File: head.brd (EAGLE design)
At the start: 15.5 x 13.2 mm, 6 parts

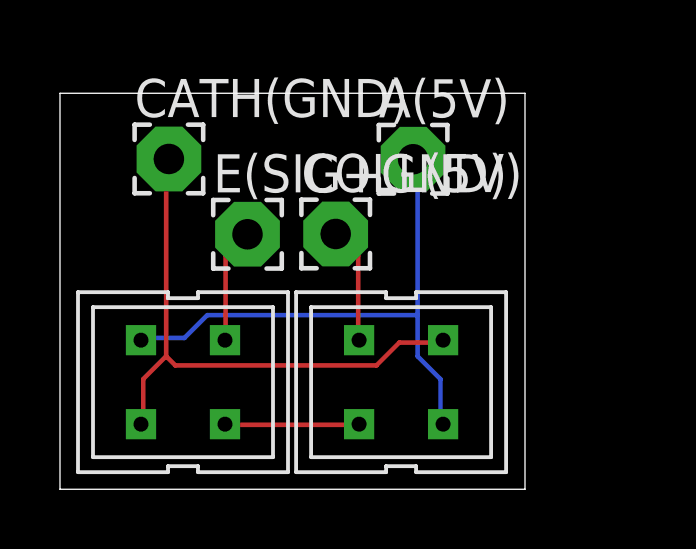
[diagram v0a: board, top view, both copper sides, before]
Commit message: no message
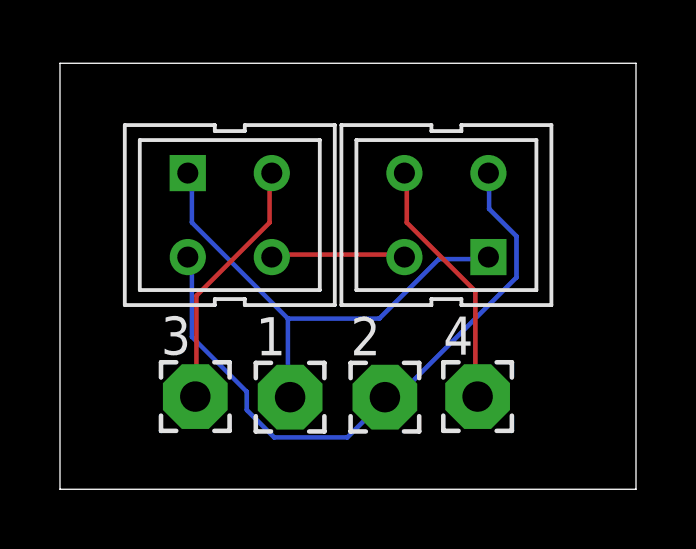
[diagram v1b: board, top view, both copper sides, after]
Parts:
- removed A(5V), CATH(GND), COLL(5V), E(SIG+GND): (no value), wirepad:2,15/1,0
- added 1, 2, 3, 4: (no value), wirepad:2,15/1,0
- moved U$2 5.78 mm to (5.66, 9.14)
- moved U$1 5.77 mm to (12.9, 9.14)
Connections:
- net A(5V): now also 1.1; no longer A(5V).1
- net CATH(GND): now also 2.1; no longer CATH(GND).1
- net COLL(5V): now also 4.1; no longer COLL(5V).1
- net E(SIG+GND): now also 3.1; no longer E(SIG+GND).1
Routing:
- net E(SIG+GND): track 3.84 -> 8.51 mm
- net COLL(5V): track 3.87 -> 8.49 mm
- net CATH(GND): track 19.0 -> 21.4 mm
- net A(5V): track 18.9 -> 16.4 mm
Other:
- board size 15.5 x 13.2 mm -> 19.2 x 14.2 mm
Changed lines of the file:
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@@
 <setting verticaltext="up"/>
 </settings>
-<grid distance="0.1" unitdist="mm" unit="mm" style="lines" multiple="1" display="yes" altdistance="1" altunitdist="mm" altunit="mm"/>
+<grid distance="0.1" unitdist="mm" unit="mm" style="lines" multiple="1" display="yes" altdistance="0.1" altunitdist="mm" altunit="mm"/>
 <layers>
 <layer number="1" name="Top" color="4" fill="1" visible="yes" active="yes"/>
@@
 <layer number="43" name="vRestrict" color="2" fill="10" visible="yes" active="yes"/>
 <layer number="44" name="Drills" color="7" fill="1" visible="no" active="yes"/>
-<layer number="45" name="Holes" color="7" fill="1" visible="yes" active="yes"/>
+<layer number="45" name="Holes" color="7" fill="1" visible="no" active="yes"/>
 <layer number="46" name="Milling" color="3" fill="1" visible="no" active="yes"/>
 <layer number="47" name="Measures" color="7" fill="1" visible="no" active="yes"/>
@@
 <board>
 <plain>
-<wire x1="0" y1="0" x2="15.5" y2="0" width="0" layer="20"/>
-<wire x1="15.5" y1="0" x2="15.5" y2="13.2" width="0" layer="20"/>
-<wire x1="15.5" y1="13.2" x2="0" y2="13.2" width="0" layer="20"/>
-<wire x1="0" y1="13.2" x2="0" y2="0" width="0" layer="20"/>
+<wire x1="0" y1="0" x2="19.2" y2="0" width="0" layer="20"/>
+<wire x1="19.2" y1="0" x2="19.2" y2="14.2" width="0" layer="20"/>
+<wire x1="19.2" y1="14.2" x2="0" y2="14.2" width="0" layer="20"/>
+<wire x1="0" y1="14.2" x2="0" y2="0" width="0" layer="20"/>
 </plain>
 <attributes>
@@
 </autorouter>
 <elements>
-<element name="A(5V)" library="wirepad" library_urn="urn:adsk.eagle:library:412" package="2,15/1,0" package3d_urn="urn:adsk.eagle:package:30831/1" value="" x="11.77" y="11"/>
-<element name="CATH(GND)" library="wirepad" library_urn="urn:adsk.eagle:library:412" package="2,15/1,0" package3d_urn="urn:adsk.eagle:package:30831/1" value="" x="3.63" y="11.01"/>
-<element name="COLL(5V)" library="wirepad" library_urn="urn:adsk.eagle:library:412" package="2,15/1,0" package3d_urn="urn:adsk.eagle:package:30831/1" value="" x="9.19" y="8.51"/>
-<element name="E(SIG+GND)" library="wirepad" library_urn="urn:adsk.eagle:library:412" package="2,15/1,0" package3d_urn="urn:adsk.eagle:package:30831/1" value="" x="6.25" y="8.5"/>
-<element name="U$1" library="ferraris_sensor_project" package="CNY70" value="CNY70" x="11.37" y="3.57" rot="R180"/>
-<element name="U$2" library="ferraris_sensor_project" package="CNY70" value="CNY70" x="4.1" y="3.57"/>
+<element name="1" library="wirepad" library_urn="urn:adsk.eagle:library:412" package="2,15/1,0" package3d_urn="urn:adsk.eagle:package:30831/1" value="" x="7.67" y="3.07"/>
+<element name="2" library="wirepad" library_urn="urn:adsk.eagle:library:412" package="2,15/1,0" package3d_urn="urn:adsk.eagle:package:30831/1" value="" x="10.83" y="3.07"/>
+<element name="3" library="wirepad" library_urn="urn:adsk.eagle:library:412" package="2,15/1,0" package3d_urn="urn:adsk.eagle:package:30831/1" value="" x="4.51" y="3.09"/>
+<element name="4" library="wirepad" library_urn="urn:adsk.eagle:library:412" package="2,15/1,0" package3d_urn="urn:adsk.eagle:package:30831/1" value="" x="13.92" y="3.09"/>
+<element name="U$1" library="ferraris_sensor_project" package="CNY70" value="CNY70" x="12.88" y="9.14" rot="R180"/>
+<element name="U$2" library="ferraris_sensor_project" package="CNY70" value="CNY70" x="5.66" y="9.14"/>
 </elements>
 <signals>
@@
 <contactref element="U$1" pad="E"/>
 <contactref element="U$2" pad="COLL"/>
-<wire x1="9.9396" y1="2.1476" x2="5.52" y2="2.1476" width="0.1524" layer="1"/>
-<wire x1="5.52" y1="2.1476" x2="5.5" y2="2.17" width="0.1524" layer="1"/>
-<wire x1="9.9396" y1="2.1476" x2="9.97" y2="2.17" width="0.1524" layer="1"/>
+<wire x1="11.4068" y1="7.824" x2="7.1396" y2="7.824" width="0.1524" layer="1"/>
+<wire x1="7.1396" y1="7.824" x2="7.06" y2="7.74" width="0.1524" layer="1"/>
+<wire x1="11.4068" y1="7.824" x2="11.48" y2="7.74" width="0.1524" layer="1"/>
 </signal>
 <signal name="CATH(GND)">
 <contactref element="U$2" pad="CATH"/>
-<contactref element="CATH(GND)" pad="1"/>
+<contactref element="2" pad="1"/>
 <contactref element="U$1" pad="CATH"/>
-<wire x1="2.7768" y1="3.6716" x2="2.7768" y2="2.3" width="0.1524" layer="1"/>
-<wire x1="3.5388" y1="4.4336" x2="2.7768" y2="3.6716" width="0.1524" layer="1"/>
-<wire x1="3.5388" y1="10.9868" x2="3.5388" y2="4.4336" width="0.1524" layer="1"/>
-<wire x1="2.7768" y1="2.3" x2="2.7" y2="2.17" width="0.1524" layer="1"/>
-<wire x1="3.5388" y1="10.9868" x2="3.63" y2="11.01" width="0.1524" layer="1"/>
-<wire x1="11.3112" y1="4.8908" x2="12.6828" y2="4.8908" width="0.1524" layer="1"/>
-<wire x1="10.5492" y1="4.1288" x2="11.3112" y2="4.8908" width="0.1524" layer="1"/>
-<wire x1="3.8436" y1="4.1288" x2="10.5492" y2="4.1288" width="0.1524" layer="1"/>
-<wire x1="3.5388" y1="4.4336" x2="3.8436" y2="4.1288" width="0.1524" layer="1"/>
-<wire x1="12.6828" y1="4.8908" x2="12.77" y2="4.97" width="0.1524" layer="1"/>
+<wire x1="4.3964" y1="5.0808" x2="4.3964" y2="7.6716" width="0.1524" layer="16"/>
+<wire x1="6.2252" y1="3.252" x2="4.3964" y2="5.0808" width="0.1524" layer="16"/>
+<wire x1="6.2252" y1="2.6424" x2="6.2252" y2="3.252" width="0.1524" layer="16"/>
+<wire x1="7.1396" y1="1.728" x2="6.2252" y2="2.6424" width="0.1524" layer="16"/>
+<wire x1="9.578" y1="1.728" x2="7.1396" y2="1.728" width="0.1524" layer="16"/>
+<wire x1="10.7972" y1="2.9472" x2="9.578" y2="1.728" width="0.1524" layer="16"/>
+<wire x1="4.3964" y1="7.6716" x2="4.26" y2="7.74" width="0.1524" layer="16"/>
+<wire x1="10.7972" y1="2.9472" x2="10.83" y2="3.07" width="0.1524" layer="16"/>
+<wire x1="14.3024" y1="9.348" x2="14.3024" y2="10.4148" width="0.1524" layer="16"/>
+<wire x1="15.2168" y1="8.4336" x2="14.3024" y2="9.348" width="0.1524" layer="16"/>
+<wire x1="15.2168" y1="7.062" x2="15.2168" y2="8.4336" width="0.1524" layer="16"/>
+<wire x1="11.2544" y1="3.0996" x2="15.2168" y2="7.062" width="0.1524" layer="16"/>
+<wire x1="10.9496" y1="3.0996" x2="11.2544" y2="3.0996" width="0.1524" layer="16"/>
+<wire x1="14.3024" y1="10.4148" x2="14.28" y2="10.54" width="0.1524" layer="16"/>
+<wire x1="10.9496" y1="3.0996" x2="10.83" y2="3.07" width="0.1524" layer="16"/>
 </signal>
 <signal name="COLL(5V)">
 <contactref element="U$1" pad="COLL"/>
-<contactref element="COLL(5V)" pad="1"/>
-<wire x1="9.9396" y1="7.7864" x2="9.9396" y2="5.0432" width="0.1524" layer="1"/>
-<wire x1="9.33" y1="8.396" x2="9.9396" y2="7.7864" width="0.1524" layer="1"/>
-<wire x1="9.9396" y1="5.0432" x2="9.97" y2="4.97" width="0.1524" layer="1"/>
-<wire x1="9.33" y1="8.396" x2="9.19" y2="8.51" width="0.1524" layer="1"/>
+<contactref element="4" pad="1"/>
+<wire x1="11.5592" y1="8.8908" x2="11.5592" y2="10.4148" width="0.1524" layer="1"/>
+<wire x1="13.8452" y1="6.6048" x2="11.5592" y2="8.8908" width="0.1524" layer="1"/>
+<wire x1="13.8452" y1="3.0996" x2="13.8452" y2="6.6048" width="0.1524" layer="1"/>
+<wire x1="11.5592" y1="10.4148" x2="11.48" y2="10.54" width="0.1524" layer="1"/>
+<wire x1="13.8452" y1="3.0996" x2="13.92" y2="3.09" width="0.1524" layer="1"/>
 </signal>
 <signal name="E(SIG+GND)">
 <contactref element="U$2" pad="E"/>
-<contactref element="E(SIG+GND)" pad="1"/>
-<wire x1="5.52" y1="7.7864" x2="5.52" y2="5.0432" width="0.1524" layer="1"/>
-<wire x1="6.1296" y1="8.396" x2="5.52" y2="7.7864" width="0.1524" layer="1"/>
-<wire x1="5.52" y1="5.0432" x2="5.5" y2="4.97" width="0.1524" layer="1"/>
-<wire x1="6.1296" y1="8.396" x2="6.25" y2="8.5" width="0.1524" layer="1"/>
+<contactref element="3" pad="1"/>
+<wire x1="6.9872" y1="8.8908" x2="6.9872" y2="10.4148" width="0.1524" layer="1"/>
+<wire x1="4.5488" y1="6.4524" x2="6.9872" y2="8.8908" width="0.1524" layer="1"/>
+<wire x1="4.5488" y1="3.0996" x2="4.5488" y2="6.4524" width="0.1524" layer="1"/>
+<wire x1="6.9872" y1="10.4148" x2="7.06" y2="10.54" width="0.1524" layer="1"/>
+<wire x1="4.5488" y1="3.0996" x2="4.51" y2="3.09" width="0.1524" layer="1"/>
 </signal>
 <signal name="A(5V)">
-<contactref element="A(5V)" pad="1"/>
+<contactref element="1" pad="1"/>
 <contactref element="U$2" pad="A"/>
 <contactref element="U$1" pad="A"/>
-<wire x1="12.6828" y1="3.6716" x2="12.6828" y2="2.3" width="0.1524" layer="16"/>
-<wire x1="11.9208" y1="4.4336" x2="12.6828" y2="3.6716" width="0.1524" layer="16"/>
-<wire x1="11.9208" y1="10.9868" x2="11.9208" y2="5.8052" width="0.1524" layer="16"/>
-<wire x1="11.9208" y1="5.8052" x2="11.9208" y2="4.4336" width="0.1524" layer="16"/>
-<wire x1="12.6828" y1="2.3" x2="12.77" y2="2.17" width="0.1524" layer="16"/>
-<wire x1="11.9208" y1="10.9868" x2="11.77" y2="11" width="0.1524" layer="16"/>
-<wire x1="4.1484" y1="5.0432" x2="2.7768" y2="5.0432" width="0.1524" layer="16"/>
-<wire x1="4.9104" y1="5.8052" x2="4.1484" y2="5.0432" width="0.1524" layer="16"/>
-<wire x1="11.9208" y1="5.8052" x2="4.9104" y2="5.8052" width="0.1524" layer="16"/>
-<wire x1="2.7768" y1="5.0432" x2="2.7" y2="4.97" width="0.1524" layer="16"/>
+<wire x1="4.3964" y1="8.8908" x2="4.3964" y2="10.4148" width="0.1524" layer="16"/>
+<wire x1="7.5968" y1="5.6904" x2="4.3964" y2="8.8908" width="0.1524" layer="16"/>
+<wire x1="7.5968" y1="3.0996" x2="7.5968" y2="5.6904" width="0.1524" layer="16"/>
+<wire x1="4.3964" y1="10.4148" x2="4.26" y2="10.54" width="0.1524" layer="16"/>
+<wire x1="7.5968" y1="3.0996" x2="7.67" y2="3.07" width="0.1524" layer="16"/>
+<wire x1="12.626" y1="7.6716" x2="14.15" y2="7.6716" width="0.1524" layer="16"/>
+<wire x1="10.6448" y1="5.6904" x2="12.626" y2="7.6716" width="0.1524" layer="16"/>
+<wire x1="7.5968" y1="5.6904" x2="10.6448" y2="5.6904" width="0.1524" layer="16"/>
+<wire x1="14.15" y1="7.6716" x2="14.28" y2="7.74" width="0.1524" layer="16"/>
 </signal>
 </signals>
